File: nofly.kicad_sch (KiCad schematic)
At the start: 8 parts, among them J1 TYPE-C-31-M-12, J2 Conn_01x04_MountingPin, U1 USBLC6-2P6

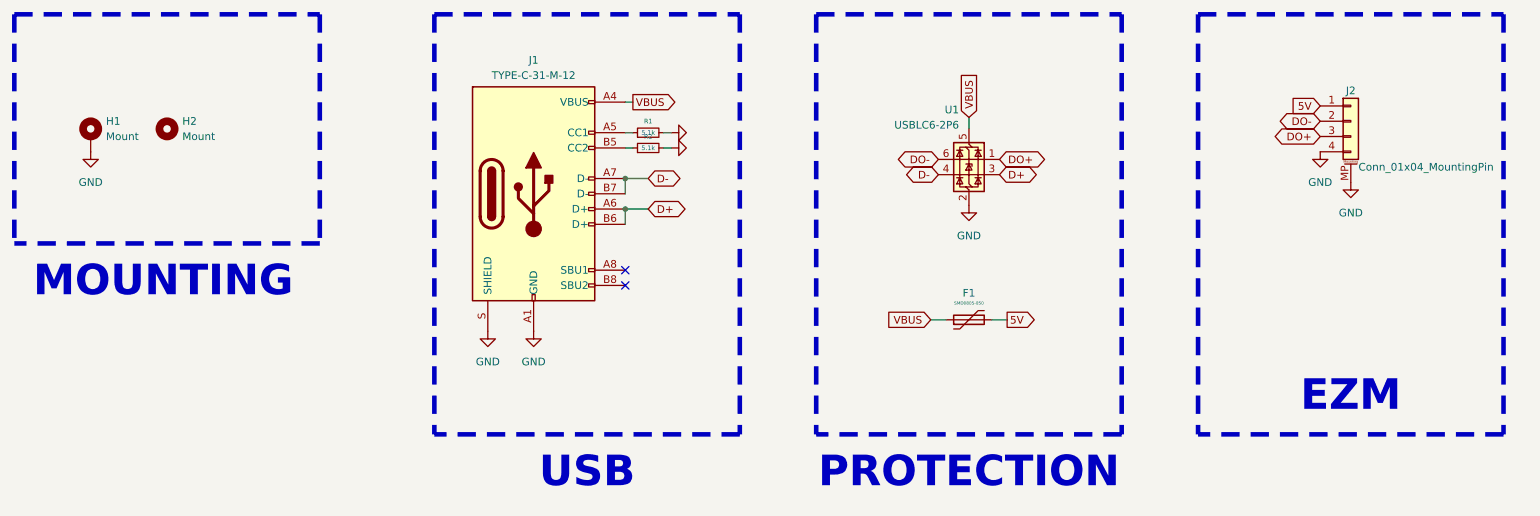
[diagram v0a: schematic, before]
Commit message: Some rerouting and checks
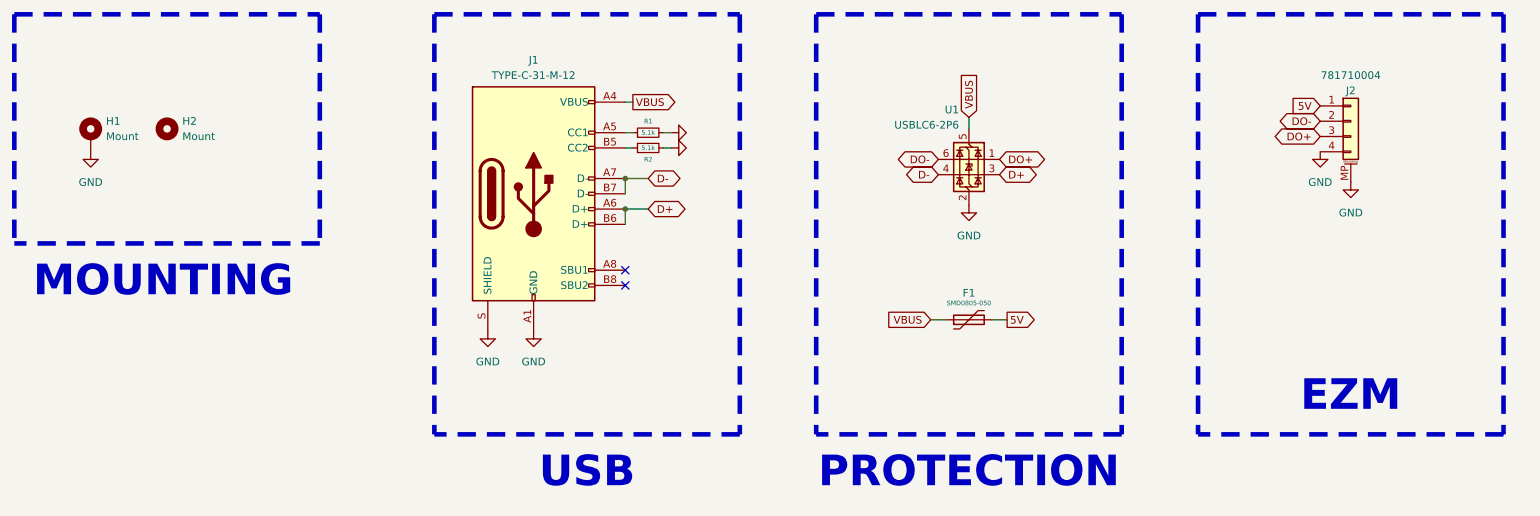
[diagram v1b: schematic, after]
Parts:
- J2: value Conn_01x04_MountingPin -> 781710004
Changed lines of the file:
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@@
 		(dnp no)
 		(property "Reference" "R2"
-			(at 130.81 39.37 90)
+			(at 130.81 43.18 90)
 			(show_name no)
 			(do_not_autoplace no)
@@
 			(effects
 				(font
-					(size 0.508 0.508)
+					(size 0.762 0.762)
 				)
 			)
@@
 			)
 		)
-		(property "Value" "Conn_01x04_MountingPin"
-			(at 248.92 44.45 0)
-			(show_name no)
-			(do_not_autoplace no)
-			(effects
-				(font
-					(size 1.27 1.27)
-				)
-				(justify left)
-			)
-		)
+		(property "Value" "781710004"
+			(at 247.65 29.21 0)
+			(show_name no)
+			(do_not_autoplace no)
+			(effects
+				(font
+					(size 1.27 1.27)
+				)
+			)
+		)
